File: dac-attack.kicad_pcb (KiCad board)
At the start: 2 copper layers, 31.1 x 43.8 mm, 59 parts, among them J1 BOARD, J2 BOARD, J3 BOARD, J4 ANALOG, J5 DIGITAL, J6 USER, J7 BTN, U1 CS8416-xZZ, U2 PCM5100, U3 SD6210A, U4 XC6206P332MR, U5 XC6206P332MR

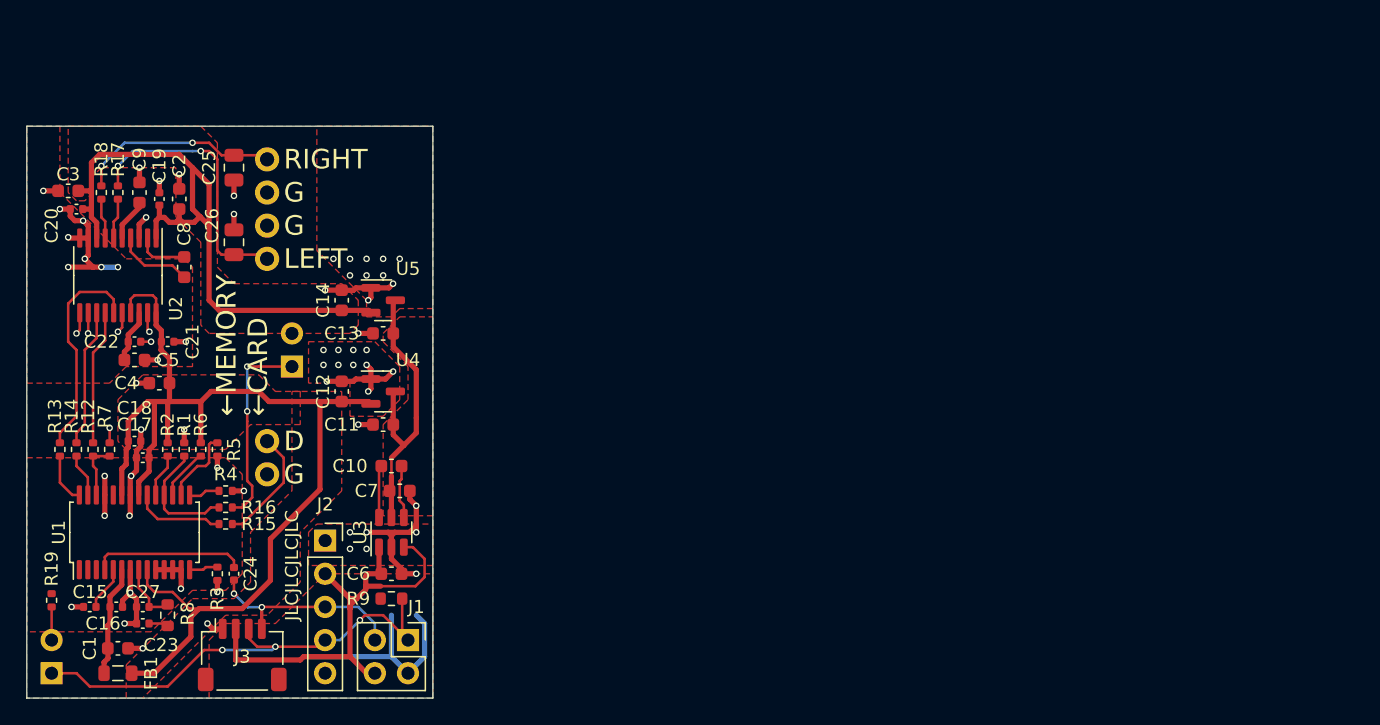
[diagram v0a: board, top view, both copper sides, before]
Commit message: Initial work on revision 2023b.
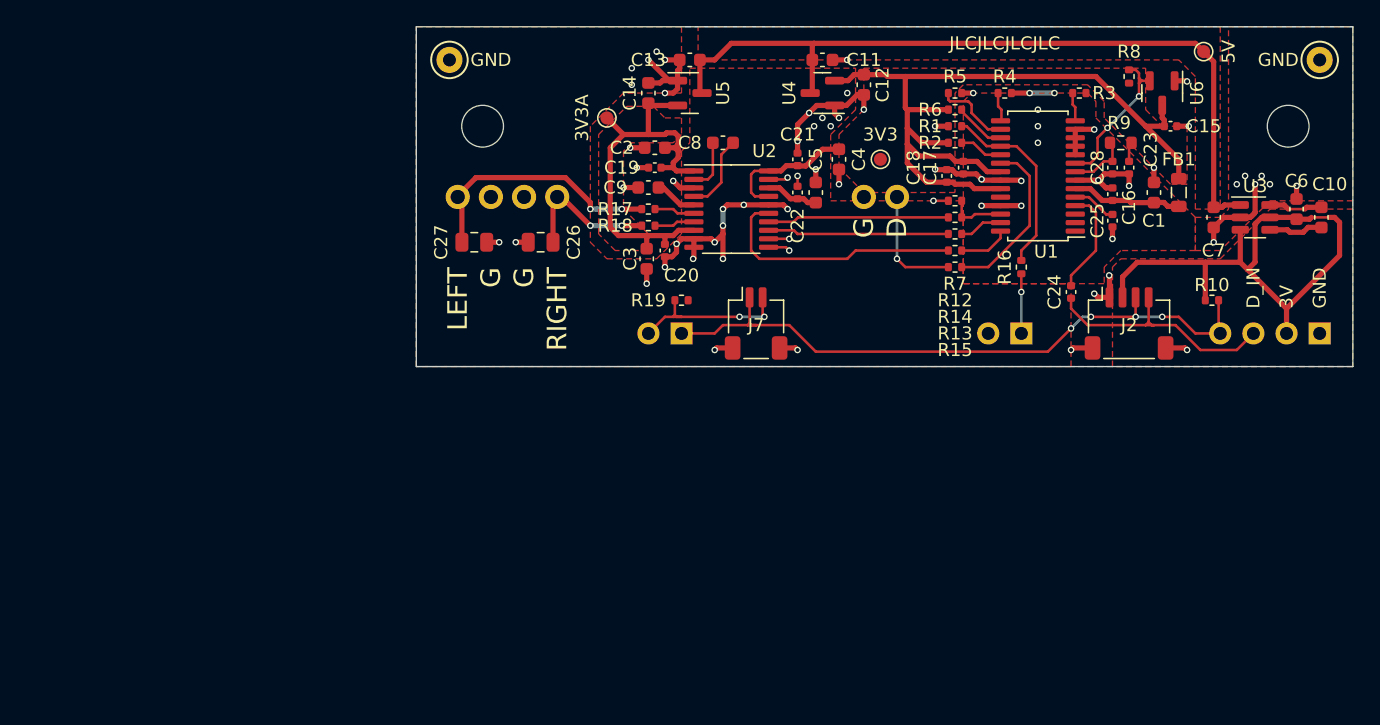
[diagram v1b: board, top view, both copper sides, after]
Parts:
- removed the J2 at (95.2, 104.1)
- removed the J6 at (92.7, 90.8)
- removed the R9 at (100.3, 108.6)
- added C25: 22nF, Capacitor_SMD:C_0402_1005Metric, F.Cu at (155.6, 79.6)
- added H1: MountingHole, MountingHole:MountingHole_3.2mm_M3, F.Cu at (107.3, 72.4)
- added H2: MountingHole, MountingHole:MountingHole_3.2mm_M3, F.Cu at (169.0, 72.4)
- added J5: USER, Connector_PinHeader_2.54mm:PinHeader_1x02_P2.54mm_Vertical, B.Cu at (148.6, 88.3)
- added J7: BTN, Connector_JST:JST_SH_SM02B-SRSS-TB_1x02-1MP_P1.00mm_Horizontal, F.Cu at (128.3, 87.5)
- added R10: 10K, Resistor_SMD:R_0402_1005Metric, F.Cu at (163.2, 85.7)
- added R8: 47K, Resistor_SMD:R_0402_1005Metric, F.Cu at (156.8, 68.6)
- added TP1: GND, TestPoint:TestPoint_Keystone_5000-5004_Miniature, F.Cu at (104.8, 67.3)
- added TP2: GND, TestPoint:TestPoint_Keystone_5000-5004_Miniature, F.Cu at (171.4, 67.3)
- added TP3: 5V, TestPoint:TestPoint_Pad_D1.0mm, F.Cu at (162.6, 66.7)
- added TP4: 3V3, TestPoint:TestPoint_Pad_D1.0mm, F.Cu at (137.8, 74.9)
- added TP5: 3V3A, TestPoint:TestPoint_Pad_D1.0mm, F.Cu at (116.8, 71.8)
- added U6: TCM809, Package_TO_SOT_SMD:SOT-23, F.Cu at (159.4, 69.8)
- J1: footprint Connector_PinSocket_2.54mm:PinSocket_2x02_P2.54mm_Vertical -> Connector_PinHeader_2.54mm:PinHeader_1x04_P2.54mm_Vertical; moved to B.Cu
- moved C15 90.6 mm to (160.0, 72.4)
- moved FB1 89.2 mm to (160.7, 77.5), turned to -90 degrees
- moved C1 86.7 mm to (158.8, 77.5), turned to 90 degrees
- moved C23 83.2 mm to (156.8, 75.6), turned to -90 degrees
- moved C16 82.6 mm to (155.6, 77.6), turned to 90 degrees
- moved C28 81.6 mm to (155.6, 75.6), turned to -90 degrees
- moved R9 81.5 mm to (156.2, 73.7), turned to 180 degrees
- moved R3 75.6 mm to (153.0, 69.8), turned to 180 degrees
- moved C6 74.8 mm to (169.7, 78.7), turned to 90 degrees
- moved U1 74.4 mm to (149.9, 76.2), turned to 180 degrees
- moved C10 73.8 mm to (171.6, 79.4), turned to 90 degrees
- moved J1 73.7 mm to (171.4, 88.3), turned to 90 degrees
- moved J2 72.5 mm to (156.8, 87.5)
- moved G*** 72.0 mm to (153.0, 72.4)
- moved U3 70.4 mm to (166.5, 79.4), turned to 0 degrees
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- renumbered C25 to C26, C26 to C27, C27 to C28, J3 to J2, J4 to J3, J5 to J4, J7 to J6, R8 to R9
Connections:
- net /DDAT renamed /D_OUT
- C15 pad 1: GND -> +3V3
- C15 pad 2: Net-(C15-Pad2) -> GND
- C24 pad 1: /DOUT -> /D_IN
- J1 pad 1: /BUTTON -> GND
- J1 pad 2: /DOUT -> /VIN
- J1 pad 3: GND -> /D_IN
- J1 pad 4: /VIN -> /BUTTON
- J2 pad 4: /DOUT -> /D_IN
- J2 pad MP: unconnected-(J3-PadMP) -> GND
- U1 pad 5: Net-(C15-Pad2) -> Net-(C25-Pad2)
- U1 pad 9: +3V3 -> Net-(R8-Pad2)
- U3 pad 1: /VIN -> +5V
- U3 pad 5: +5V -> /VIN
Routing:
- net +5V: track 22.9 -> 60.3 mm
- net /D_IN: track 0.00 -> 19.3 mm
- net /DOUT: track 18.6 -> 0.00 mm, vias 2 -> 0
- net +3.3VA: track 52.1 -> 33.6 mm
- net /BUTTON: track 37.2 -> 50.8 mm, vias 3 -> 4
- net +3V3: track 87.0 -> 73.7 mm
- net Net-(R8-Pad2): track 0.00 -> 11.7 mm, vias 0 -> 2
- net /USER: track 15.5 -> 4.57 mm, vias 2 -> 1
- net Net-(J7-Pad2): track 2.54 -> 12.8 mm, vias 0 -> 2
- net /VIN: track 35.9 -> 42.4 mm
- net Net-(R15-Pad1): track 7.03 -> 13.0 mm
- net Net-(R1-Pad1): track 9.21 -> 14.7 mm
- net /RIGHT: track 15.5 -> 11.3 mm
- net /ADAT: track 10.3 -> 13.9 mm
- net Net-(C24-Pad2): track 11.7 -> 8.20 mm
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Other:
- board size 31.1 x 43.8 mm -> 71.8 x 26 mm
- board text added: "3V"
- board text added: "B_READ"
- board text added: "D_IN"
- board text added: "EXT BUTTON"
- board text added: "GND"
- board text added: "Rev 2023b Licensed under CERN-OHL-S v2"
- board text removed: "BTN"
- board text removed: "Rev 2023a Licensed under CERN-OHL-S v2"
- board text removed: "←MEMORY ←CARD"
